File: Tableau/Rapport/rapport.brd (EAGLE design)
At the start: 105 x 91 mm, 22 parts

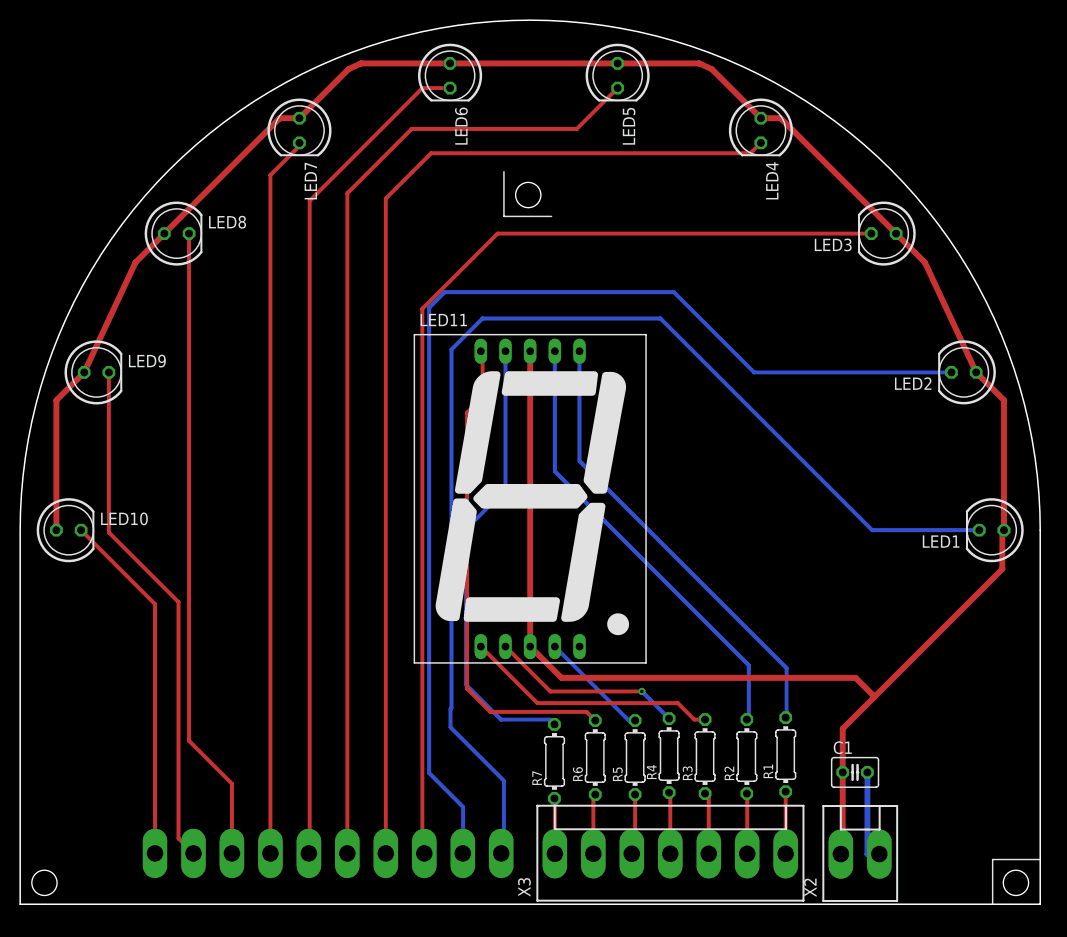
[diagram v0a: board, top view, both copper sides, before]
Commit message: no message
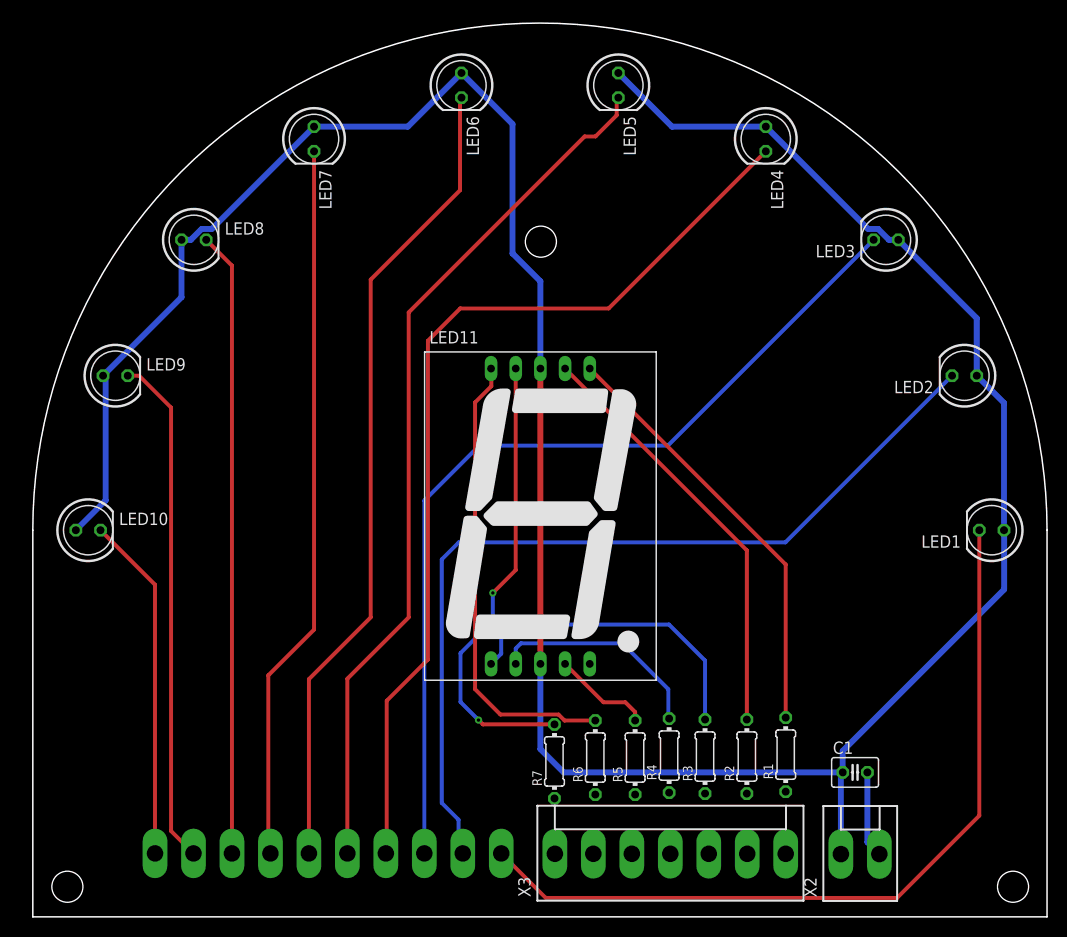
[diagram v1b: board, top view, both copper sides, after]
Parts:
- moved LED11 2.07 mm to (221.1, 91.4)
- moved LED10 2.00 mm to (174.5, 90.0)
- moved LED9 1.97 mm to (177.3, 105.9)
- moved LED8 1.88 mm to (185.4, 119.9)
- moved LED7 1.73 mm to (197.8, 130.3)
- moved LED6 1.53 mm to (212.9, 135.8)
- moved LED4 1.00 mm to (244.2, 130.3)
- moved LED5 0.99 mm to (229.1, 135.8)
- moved LED3 0.68 mm to (256.6, 119.9)
- moved LED2 0.35 mm to (264.7, 105.9)
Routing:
- net BARGRAPH_0: track 119.0 -> 84.0 mm
- net BARGRAPH_1: track 115.5 -> 92.8 mm
- net VCC: track 266.2 -> 286.4 mm
- net BARGRAPH_2: track 105.6 -> 93.7 mm
- net BARGRAPH_3: track 108.4 -> 97.4 mm
- net BARGRAPH_4: track 100.3 -> 90.0 mm
- net 7SEG_G: track 6.40 -> 0.00 mm
- net 7SEG_E: track 6.36 -> 0.00 mm
- net 7SEG_D: track 6.35 -> 0.00 mm
- net 7SEG_C: track 6.24 -> 0.00 mm
- net 7SEG_F: track 6.22 -> 0.00 mm
- net 7SEG_B: track 6.18 -> 0.00 mm
- net N$6: track 26.2 -> 32.3 mm
- net 7SEG_A: track 5.72 -> 0.00 mm
- net N$5: track 19.9 -> 22.5 mm, vias 1 -> 0
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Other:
- board size 105 x 91 mm -> 104.4 x 92 mm
